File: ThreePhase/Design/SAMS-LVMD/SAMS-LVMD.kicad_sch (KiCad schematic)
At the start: 79 parts, among them J1 SIGNALS, J2 POWER INPUT, J3 MOTOR OUTPUT, Q1 55V/42A, U1 U CHANNEL DRIVER, U2 V CHANNEL DRIVER, U3 W CHANNEL DRIVER, U4 ISEN 50mV/V, U5 ISEN 50mV/V, U6 ISEN 50mV/V

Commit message: 3P schematic update 4
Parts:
- C18, C20, C21: footprint (none) -> SAMPI:CAP_ELEC-10.3x10.3-DIA10
- D10, D11, D12, D13, D14, D15, D16, D7, D8: footprint Liem:SOD-323_12 -> SAMPI:SOD-923
- D9: footprint (none) -> SAMPI:SOD-123
- J1: footprint (none) -> SAMPI:IDC-2x7x2MM-TH
- Q1: footprint (none) -> SAMPI:D2PAK_TO-263
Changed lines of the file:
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@@
 			)
 		)
-		(property "Footprint" "Liem:SOD-323_12"
+		(property "Footprint" "SAMPI:SOD-923"
 			(at 274.955 69.85 0)
 			(effects
@@
 			)
 		)
-		(property "Footprint" "Liem:SOD-323_12"
+		(property "Footprint" "SAMPI:SOD-923"
 			(at 205.105 72.39 0)
 			(effects
@@
 			)
 		)
-		(property "Footprint" "Liem:SOD-323_12"
+		(property "Footprint" "SAMPI:SOD-923"
 			(at 217.805 72.39 0)
 			(effects
@@
 			)
 		)
-		(property "Footprint" "Liem:SOD-323_12"
+		(property "Footprint" "SAMPI:SOD-923"
 			(at 211.455 72.39 0)
 			(effects
@@
 			)
 		)
-		(property "Footprint" "Liem:SOD-323_12"
+		(property "Footprint" "SAMPI:SOD-923"
 			(at 198.755 72.39 0)
 			(effects
@@
 			)
 		)
-		(property "Footprint" ""
+		(property "Footprint" "SAMPI:CAP_ELEC-10.3x10.3-DIA10"
 			(at 204.47 101.6 0)
 			(effects
@@
 			)
 		)
-		(property "Footprint" ""
+		(property "Footprint" "SAMPI:SOD-123"
 			(at 254 106.68 0)
 			(effects
@@
 			)
 		)
-		(property "Footprint" "Liem:SOD-323_12"
+		(property "Footprint" "SAMPI:SOD-923"
 			(at 201.295 157.48 0)
 			(effects
@@
 			)
 		)
-		(property "Footprint" ""
+		(property "Footprint" "SAMPI:IDC-2x7x2MM-TH"
 			(at 231.14 50.8 0)
 			(effects
@@
 			)
 		)
-		(property "Footprint" ""
+		(property "Footprint" "SAMPI:CAP_ELEC-10.3x10.3-DIA10"
 			(at 217.17 101.6 0)
 			(effects
@@
 			)
 		)
-		(property "Footprint" ""
+		(property "Footprint" "SAMPI:CAP_ELEC-10.3x10.3-DIA10"
 			(at 229.87 101.6 0)
 			(effects
@@
 			)
 		)
-		(property "Footprint" "Liem:SOD-323_12"
+		(property "Footprint" "SAMPI:SOD-923"
 			(at 268.605 69.85 0)
 			(effects
@@
 			)
 		)
-		(property "Footprint" "Liem:SOD-323_12"
+		(property "Footprint" "SAMPI:SOD-923"
 			(at 255.905 69.85 0)
 			(effects
@@
 			)
 		)
-		(property "Footprint" ""
+		(property "Footprint" "SAMPI:D2PAK_TO-263"
 			(at 261.62 101.6 0)
 			(effects
@@
 			)
 		)
-		(property "Footprint" "Liem:SOD-323_12"
+		(property "Footprint" "SAMPI:SOD-923"
 			(at 262.255 69.85 0)
 			(effects

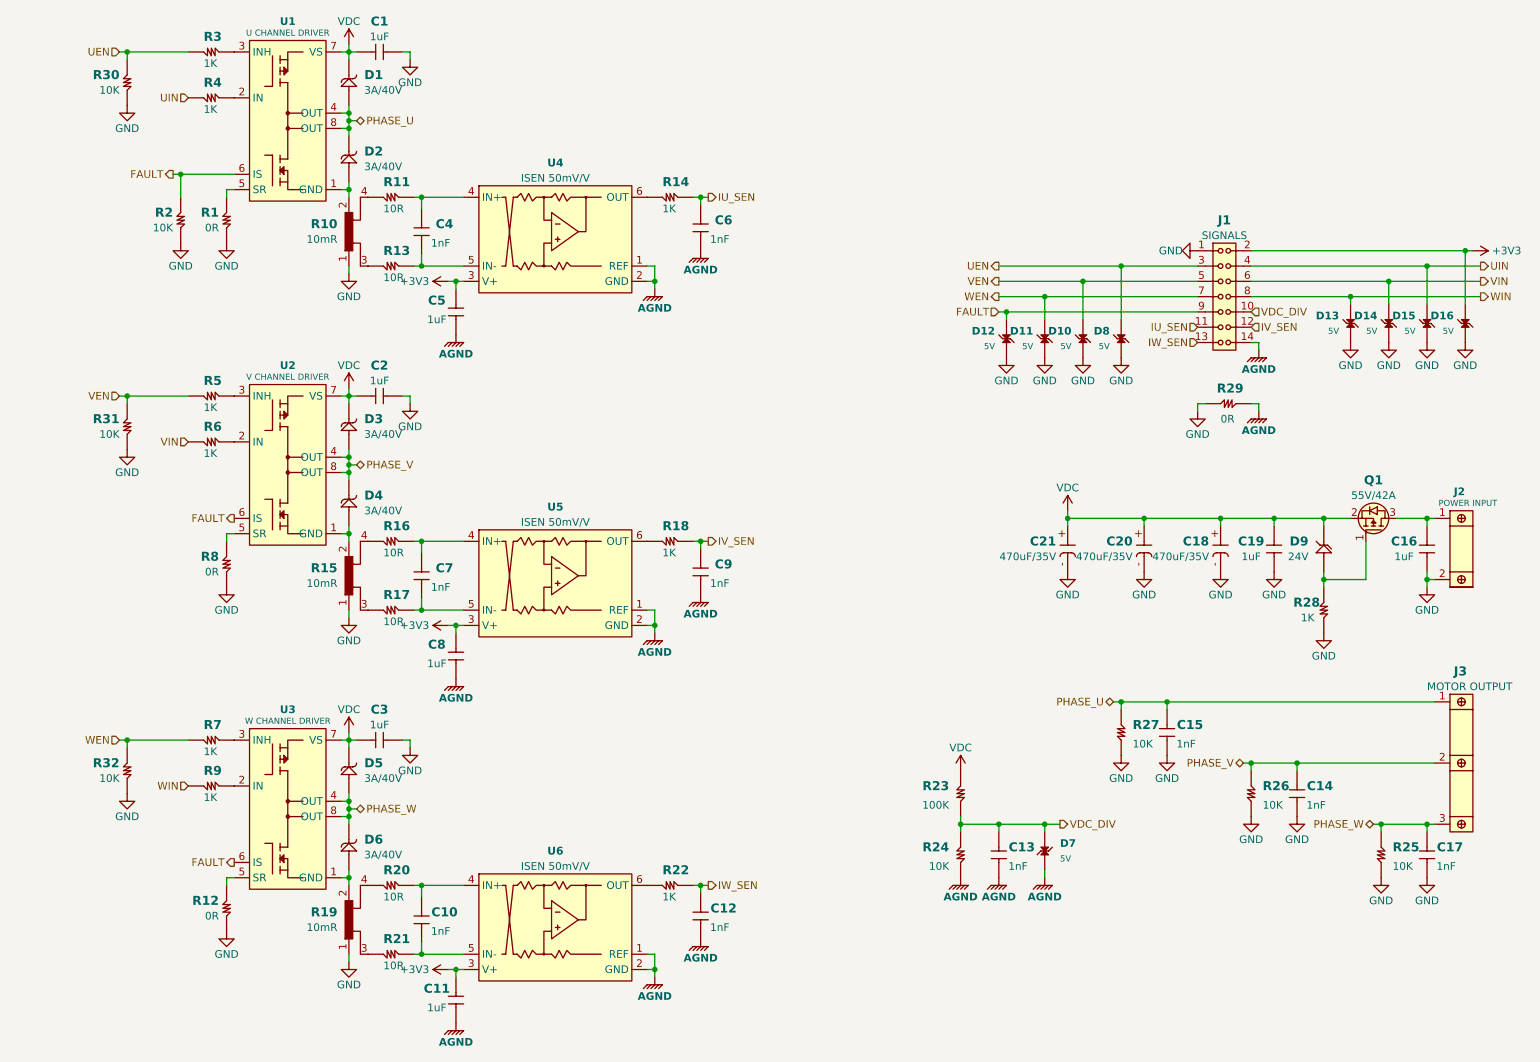
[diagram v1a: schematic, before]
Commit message: 3P schematic update 5
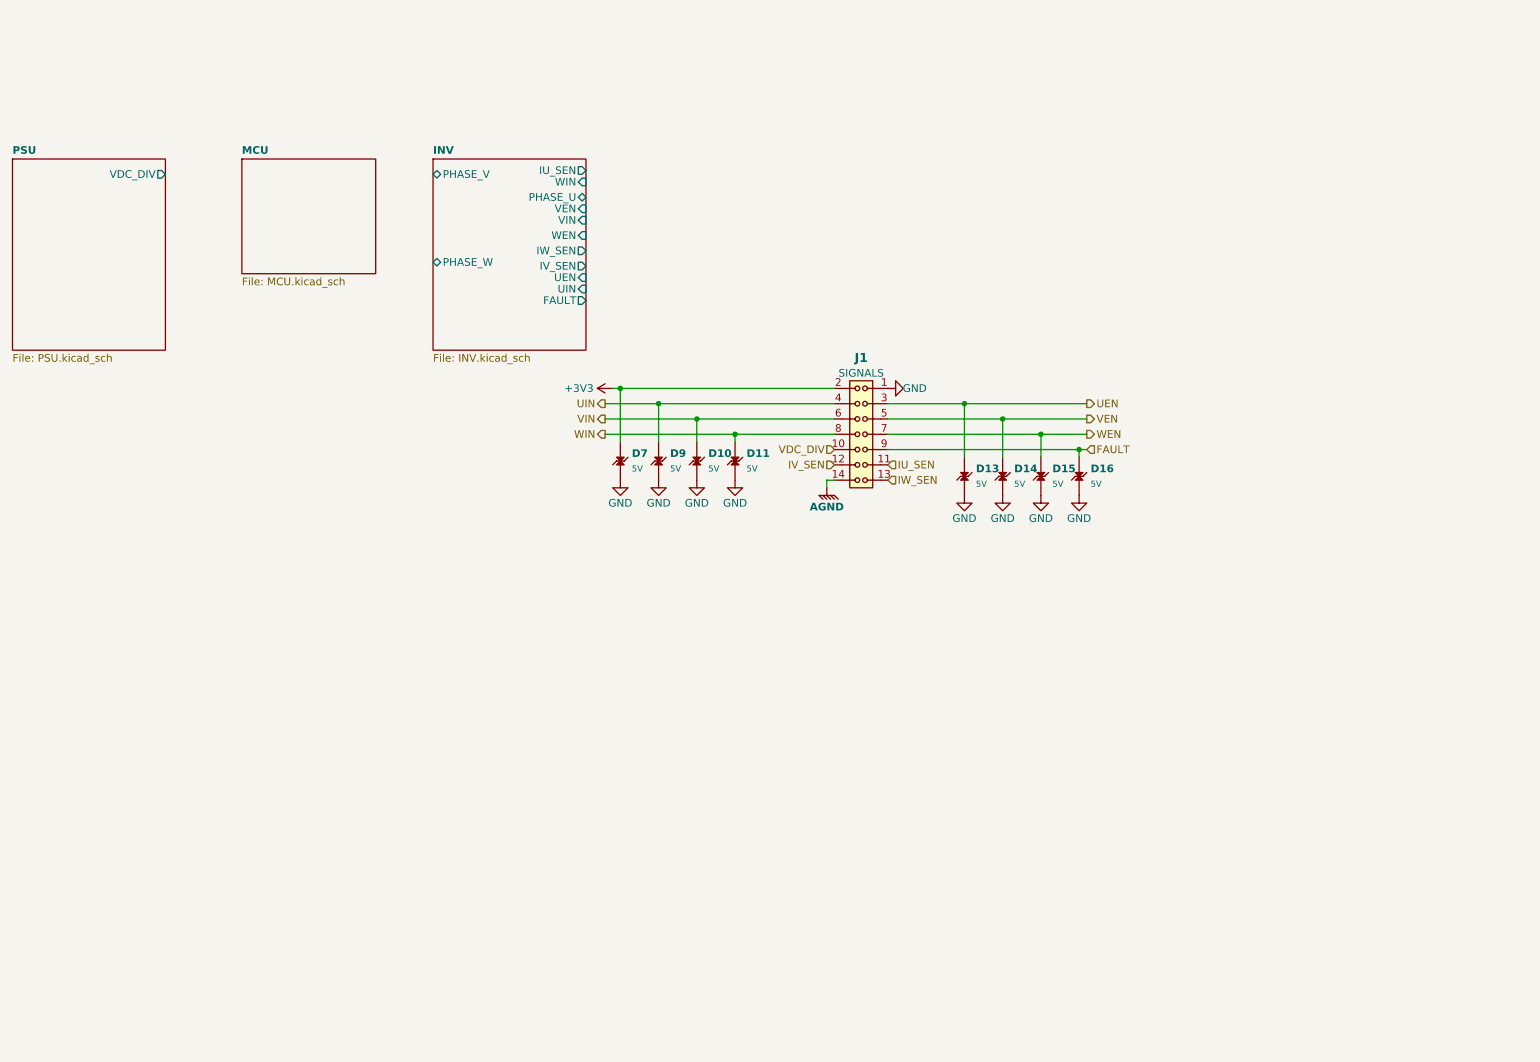
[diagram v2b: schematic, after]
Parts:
- removed C1, C11, C16, C19, C2, C3, C5, C8: 1uF, SAMPI:CAP0603, symbol SAMPI:CERCAP
- removed C10, C12, C13, C14, C15, C17, C4, C6, C7, C9: 1nF, SAMPI:CAP0603, symbol SAMPI:CERCAP
- removed C18, C20, C21: 470uF/35V, SAMPI:CAP_ELEC-10.3x10.3-DIA10, symbol SAMPI:ELECCAP
- removed D1, D2, D3, D4, D5, D6: 3A/40V, SAMPI:DO-214AB, symbol SAMPI:DIODE-SCH
- removed D12, D8: 5V, SAMPI:SOD-923, symbol SAMPI:TVS
- removed D9: 24V, SAMPI:SOD-123, symbol Liem:DIODE-ZEN
- removed J2: POWER INPUT, symbol Liem:SIL02
- removed J3: MOTOR OUTPUT, symbol SAMPI:SIL03
- removed Q1: 55V/42A, SAMPI:D2PAK_TO-263, symbol Liem:FET_P-CH
- removed R1, R12, R29, R8: 0R, SAMPI:RES0603, symbol SAMPI:RES
- removed R10, R15, R19: 10mR, SAMPI:SHUNT_1206, symbol SAMPI:SHUNT
- removed R11, R13, R16, R17, R20, R21: 10R, SAMPI:RES0603, symbol SAMPI:RES
- removed R14, R18, R22, R28, R3, R4, R5, R6, R7, R9: 1K, SAMPI:RES0603, symbol SAMPI:RES
- removed R2, R24, R25, R26, R27, R30, R31, R32: 10K, SAMPI:RES0603, symbol SAMPI:RES
- removed R23: 100K, SAMPI:RES0603, symbol SAMPI:RES
- removed U1: U CHANNEL DRIVER, SAMPI:TO-263-7, symbol SAMPI:BTS7960
- removed U2: V CHANNEL DRIVER, SAMPI:TO-263-7, symbol SAMPI:BTS7960
- removed U3: W CHANNEL DRIVER, SAMPI:TO-263-7, symbol SAMPI:BTS7960
- removed U4, U5, U6: ISEN 50mV/V, SAMPI:SOT363, symbol SAMPI:ZXCT199Q_INV
- added D9: 5V, SAMPI:SOD-923, symbol SAMPI:TVS
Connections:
- net +3V3: now also D7.1; no longer D16.1
- net AGND: no longer D7.2
- net FAULT: now also D16.1
- net GND: now also D7.2, D9.2
- net UEN: now also D13.1
- net UIN: now also D9.1; no longer D15.1
- net VDC_DIV: no longer D7.1
- net VEN: now also D14.1; no longer D10.1
- net VIN: now also D10.1; no longer D14.1
- net WEN: now also D15.1; no longer D11.1
- net WIN: now also D11.1; no longer D13.1
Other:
- added sheet INV (INV.kicad_sch)
- added sheet MCU (MCU.kicad_sch)
- added sheet PSU (PSU.kicad_sch)
